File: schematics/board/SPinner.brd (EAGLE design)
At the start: 323.2 x 241.6 mm, 8 parts

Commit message: Внутренняя плата СБ v2
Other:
- board size 323.2 x 241.6 mm -> 63.6 x 63.6 mm
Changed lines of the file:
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@@
 <board>
 <plain>
-<wire x1="-82" y1="-82" x2="241.2" y2="-82" width="0" layer="20"/>
-<wire x1="241.2" y1="-82" x2="170.6" y2="159.6" width="0" layer="20"/>
-<wire x1="170.6" y1="159.6" x2="-82" y2="150.6" width="0" layer="20"/>
-<wire x1="-82" y1="150.6" x2="-82" y2="-82" width="0" layer="20"/>
 <wire x1="9.1802" y1="65.748740625" x2="16.251259375" y2="72.819809375" width="0.001" layer="20"/>
 <wire x1="16.251259375" y1="9.1802" x2="9.1802" y2="16.251259375" width="0.001" layer="20"/>
@@
 <param name="mdViaViaSameLayer" value="6mil"/>
 <param name="mnLayersViaInSmd" value="2"/>
-<param name="mdCopperDimension" value="19mil"/>
+<param name="mdCopperDimension" value="10mil"/>
 <param name="mdDrill" value="6mil"/>
 <param name="mdSmdStop" value="0mil"/>

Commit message: Гербер SPinner
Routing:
- net BUS+1: track 82.7 -> 75.4 mm

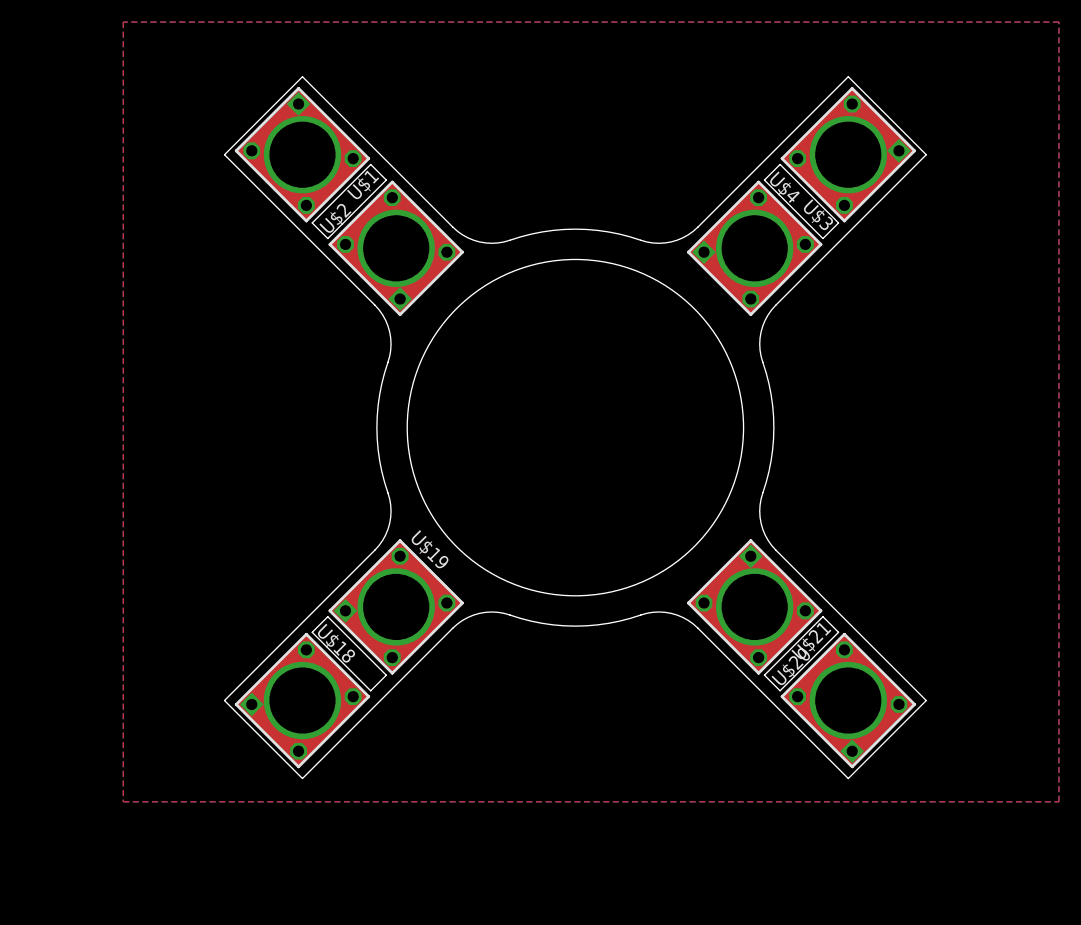
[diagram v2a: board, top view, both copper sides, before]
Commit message: Обновлен гербер SPinner
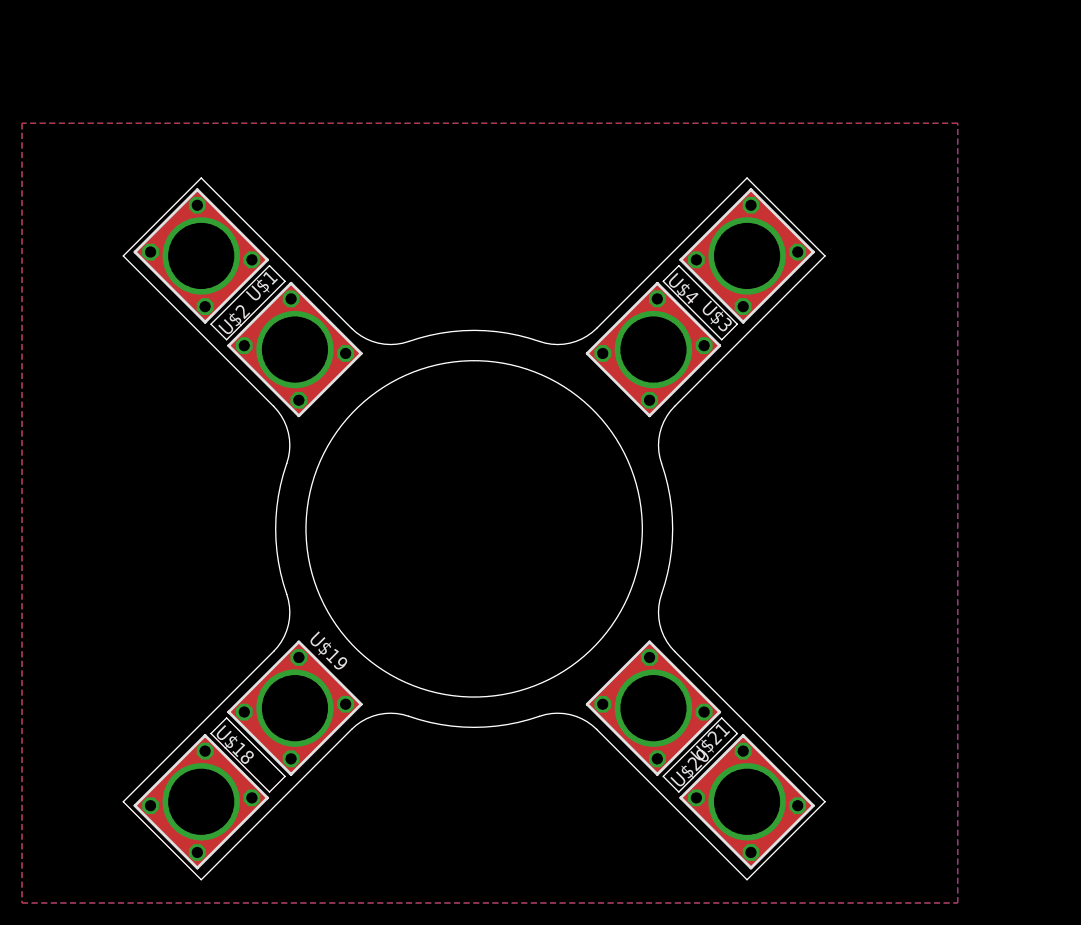
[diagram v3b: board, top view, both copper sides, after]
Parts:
- moved U$1 13.0 mm to (7.07, 56.6)
- moved U$18 13.0 mm to (7.07, 7.07)
- moved U$19 13.0 mm to (15.6, 15.6)
- moved U$2 13.0 mm to (15.6, 48.1)
- moved U$20 13.0 mm to (56.6, 7.07)
- moved U$21 13.0 mm to (48.1, 15.6)
- moved U$3 13.0 mm to (56.6, 56.6)
- moved U$4 13.0 mm to (48.1, 48.1)
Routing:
- added copper zone on layer 16, net BUS+1
- added copper zone on layer 1, net N$2
- removed copper zone on layer 1, net BUS+1
- removed copper zone on layer 16, net N$2

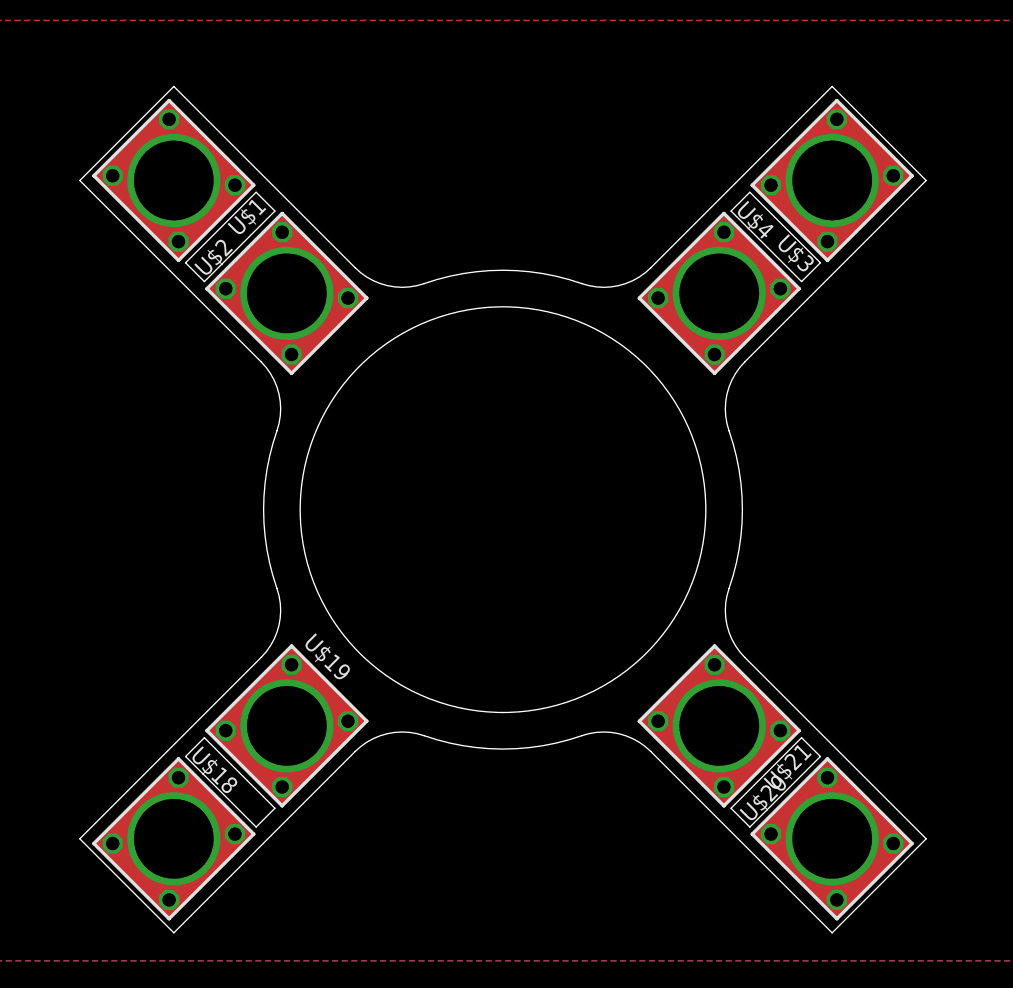
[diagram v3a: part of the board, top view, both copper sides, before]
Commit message: Обновлены герберы плат
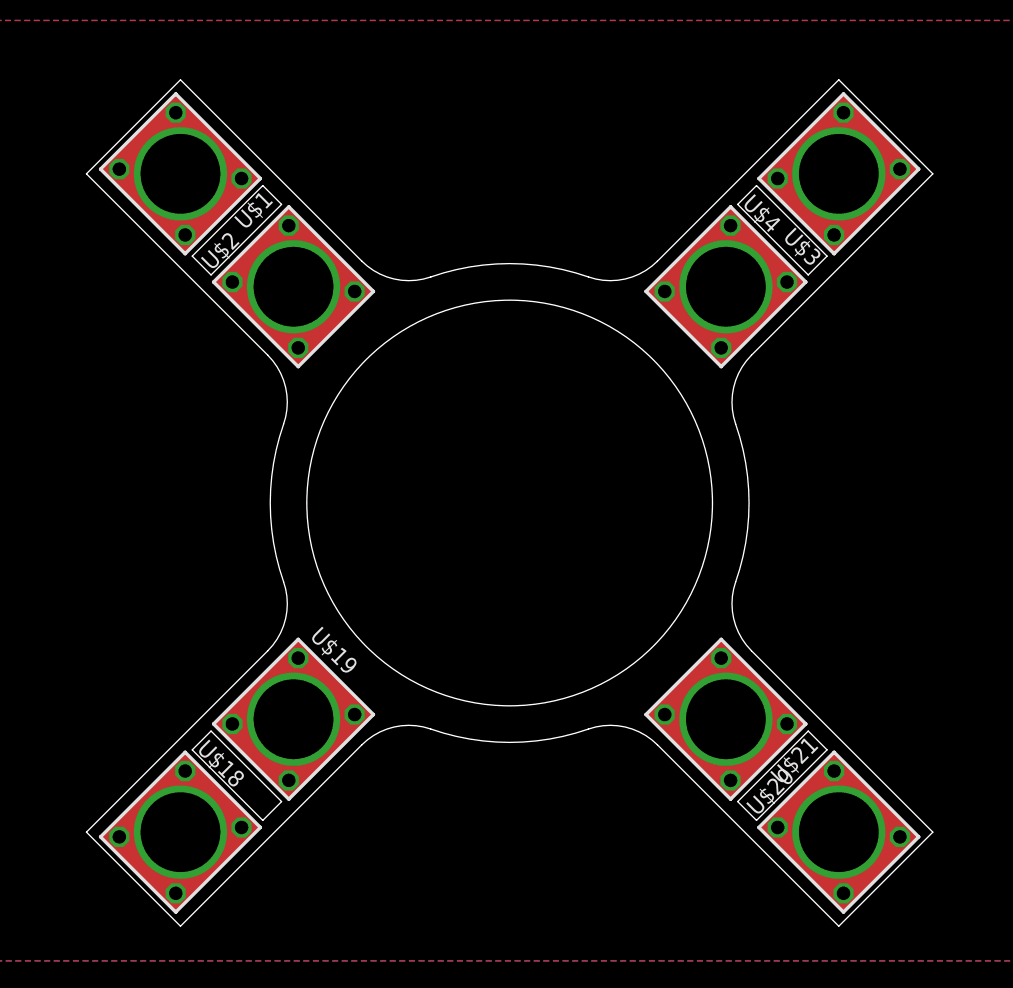
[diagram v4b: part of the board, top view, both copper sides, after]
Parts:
- moved U$1 0.71 mm to (7.57, 57.1)
- moved U$18 0.71 mm to (7.57, 7.57)
- moved U$19 0.71 mm to (16.1, 16.1)
- moved U$2 0.71 mm to (16.1, 48.6)
- moved U$20 0.71 mm to (57.1, 7.57)
- moved U$21 0.71 mm to (48.6, 16.1)
- moved U$3 0.71 mm to (57.1, 57.1)
- moved U$4 0.71 mm to (48.6, 48.6)
